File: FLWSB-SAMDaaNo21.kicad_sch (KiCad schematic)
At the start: 36 parts, among them J1 USB4085-GF-A_REVA4, J2 DEBUG, J3 Conn_01x15_Male, J4 Conn_01x15_Male, SW1 SW_RESET, U1 LD1117S33TR_SOT223, U2 ATSAMD21G18A-A, Y1 Crystal_Small

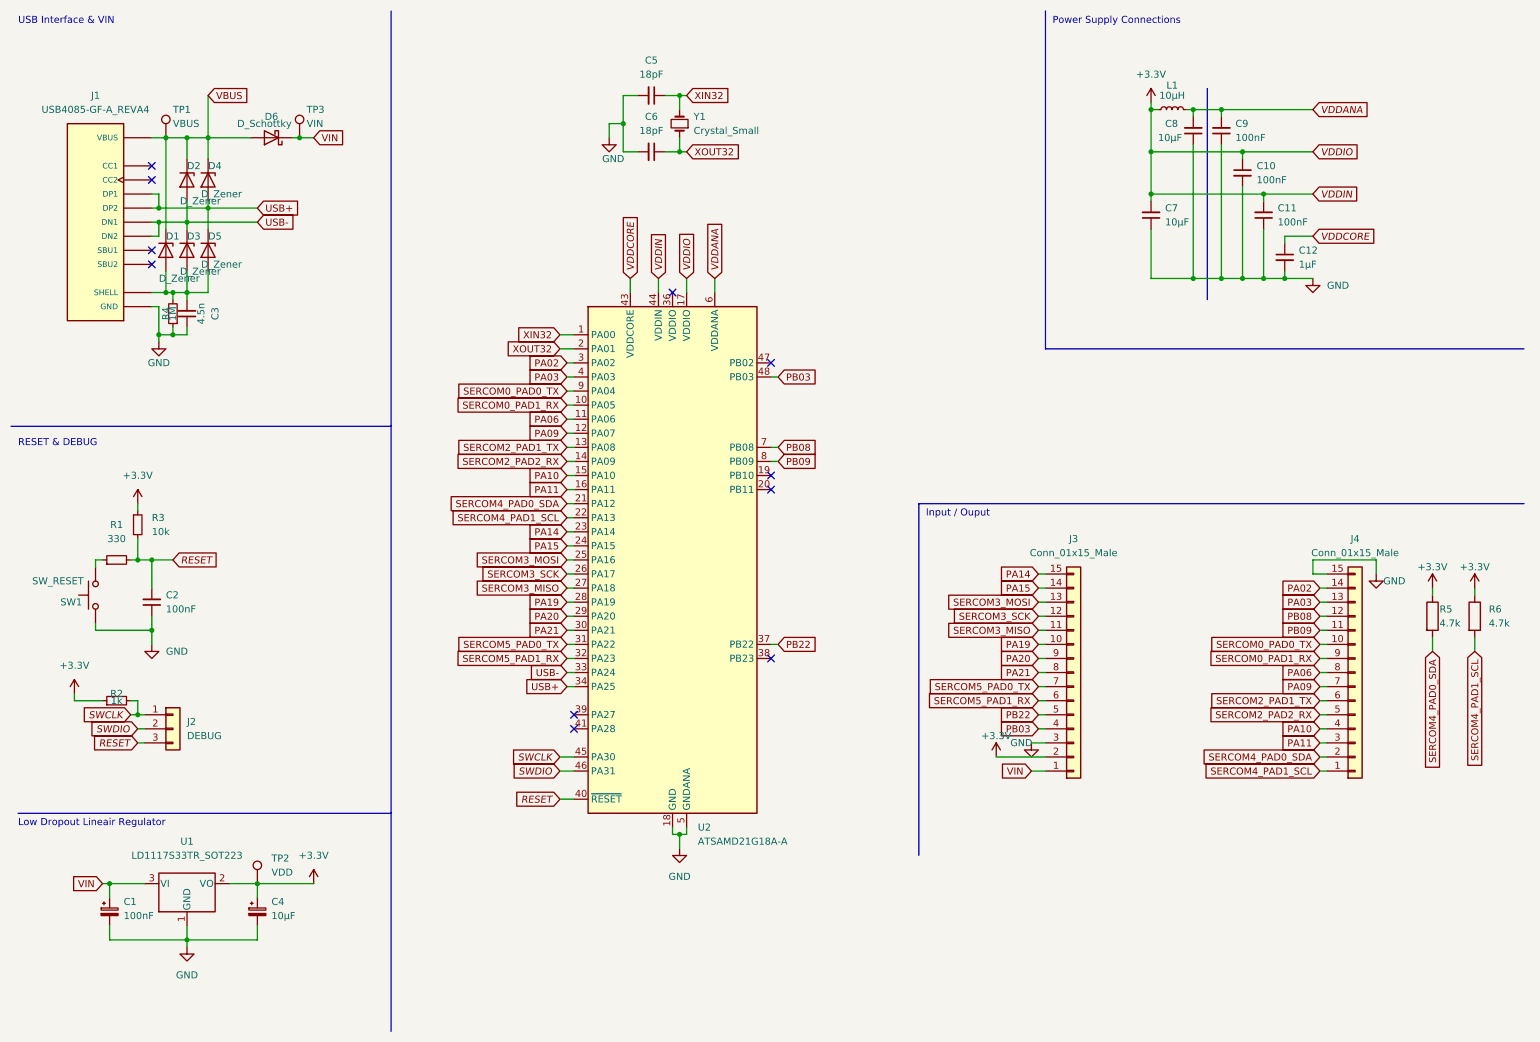
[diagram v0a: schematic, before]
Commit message: Laatste verbeteringen
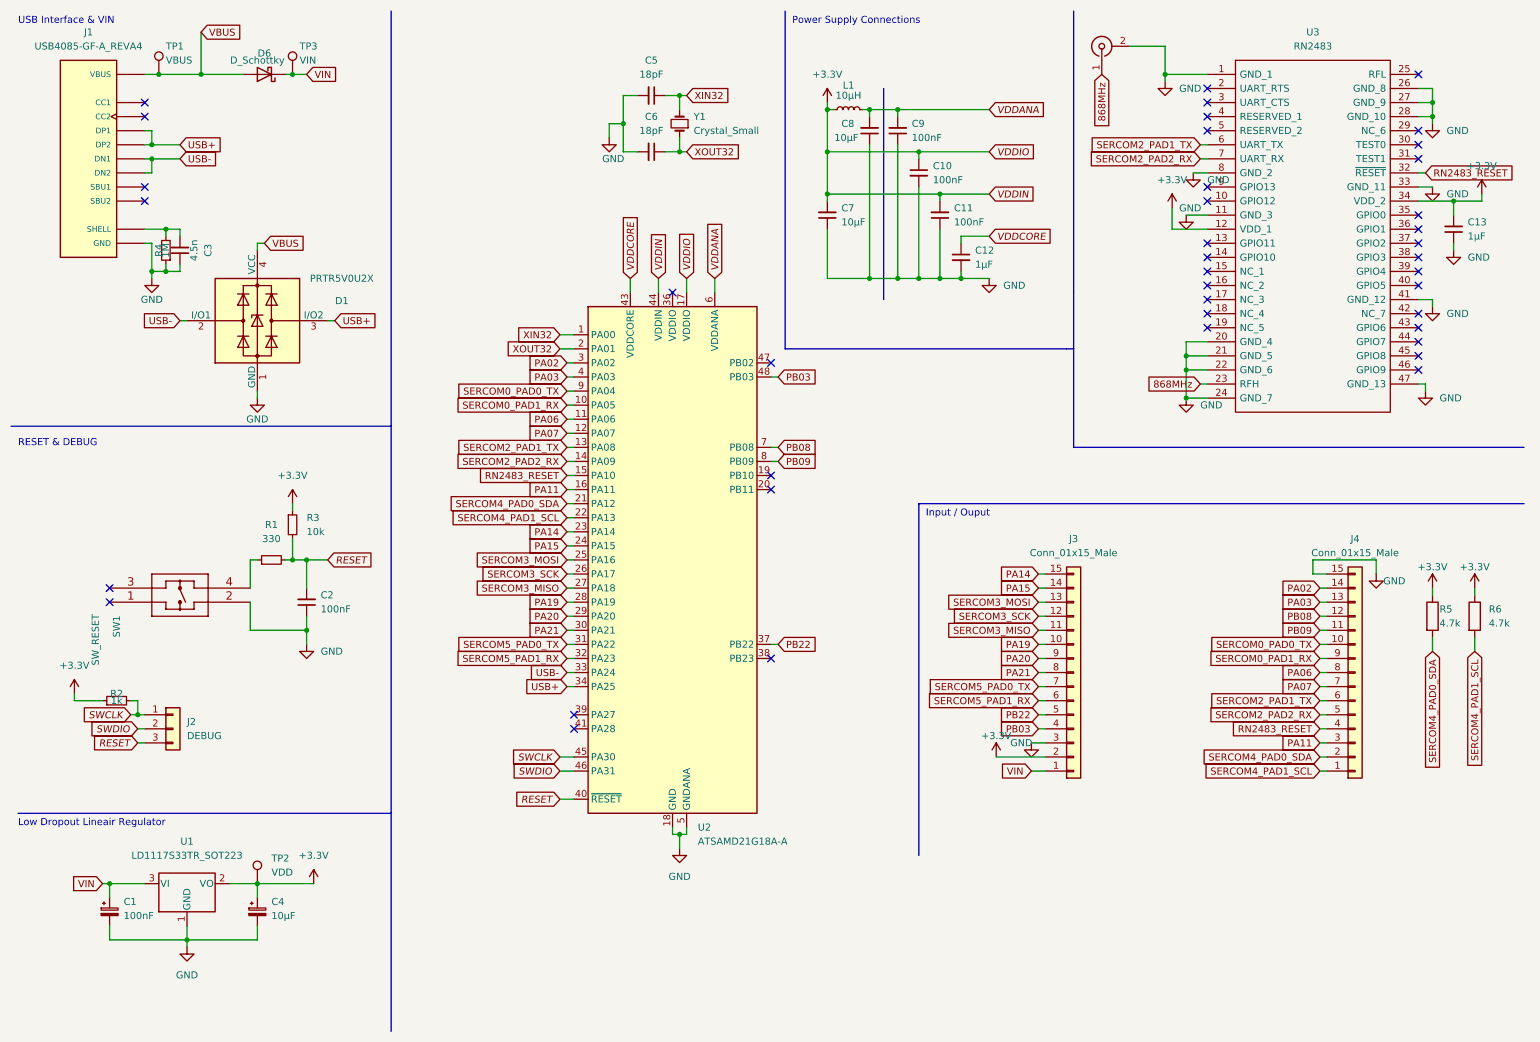
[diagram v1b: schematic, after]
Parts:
- removed D1, D2, D3, D4, D5: D_Zener, Resistor_SMD:R_0805_2012Metric_Pad1.20x1.40mm_HandSolder, symbol Device:D_Zener
- added C13: 1µF, Capacitor_SMD:C_0805_2012Metric_Pad1.18x1.45mm_HandSolder, symbol Device:C_Small
- added D1: PRTR5V0U2X, Package_TO_SOT_SMD:SOT-143, symbol Power_Protection:PRTR5V0U2X
- added J6: Conn_Coaxial, Connector_Coaxial:U.FL_Molex_MCRF_73412-0110_Vertical, symbol Connector:Conn_Coaxial
- added U3: RN2483, RN2483:RN2483, symbol RN2483:RN2483
- SW1: footprint Button_Switch_SMD:SW_Push_1P1T_NO_6x6mm_H9.5mm -> KMR7_CNK:KMR7_CNK; symbol Switch:SW_Push -> KMR221G-LFS:KMR731NGLFS
- TP1, TP2, TP3: footprint TestPoint:TestPoint_Pad_D1.0mm -> TestPoint:TestPoint_THTPad_1.0x1.0mm_Drill0.5mm
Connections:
- net +3V3: now also C13.2, U3.12 (VDD_1), U3.34 (VDD_2)
- net GND: now also C13.1, D1.1 (GND), J6.2 (Ext), U3.1 (GND_1), U3.11 (GND_3), U3.20 (GND_4), U3.21 (GND_5), U3.22 (GND_6), U3.24 (GND_7), U3.26 (GND_8), U3.27 (GND_9), U3.28 (GND_10), U3.33 (GND_11), U3.41 (GND_12), U3.47 (GND_13), U3.8 (GND_2)
- net SERCOM2_PAD1_TX: now also U3.6 (UART_TX)
- net SERCOM2_PAD2_RX: now also U3.7 (UART_RX)
- net USB+: now also D1.3 (I/O2)
- net USB-: now also D1.2 (I/O1)
- net VBUS: now also D1.4 (VCC)
- net at SW1.1: no longer R1.1
- net PA09 renamed PA07
- net PA10 renamed RN2483_RESET
- net RN2483_RESET: now also U3.32 (~{RESET})
- new net: R1.1, SW1.4
- new net 868MHz: J6.1 (In), U3.23 (RFH)
- no-connect marks 11 -> 41
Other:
- moved on the sheet: C10, C11, C12, C2, C3, C7, C8, C9, D6, J1, L1, R1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
